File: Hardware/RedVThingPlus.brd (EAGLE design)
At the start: 58.4 x 22.9 mm, 91 parts, among them J1 FEMALE 2x3, J2 USB Female Type C Connector, J5 JTAG, Q1 3.1A/30V/105mΩ, U1 MCP73831, U2 1.8V, U3 AP2112-3.3V, U4 FE310, U5 32MB, Y1 32.768KHZ, Y2 16MHz

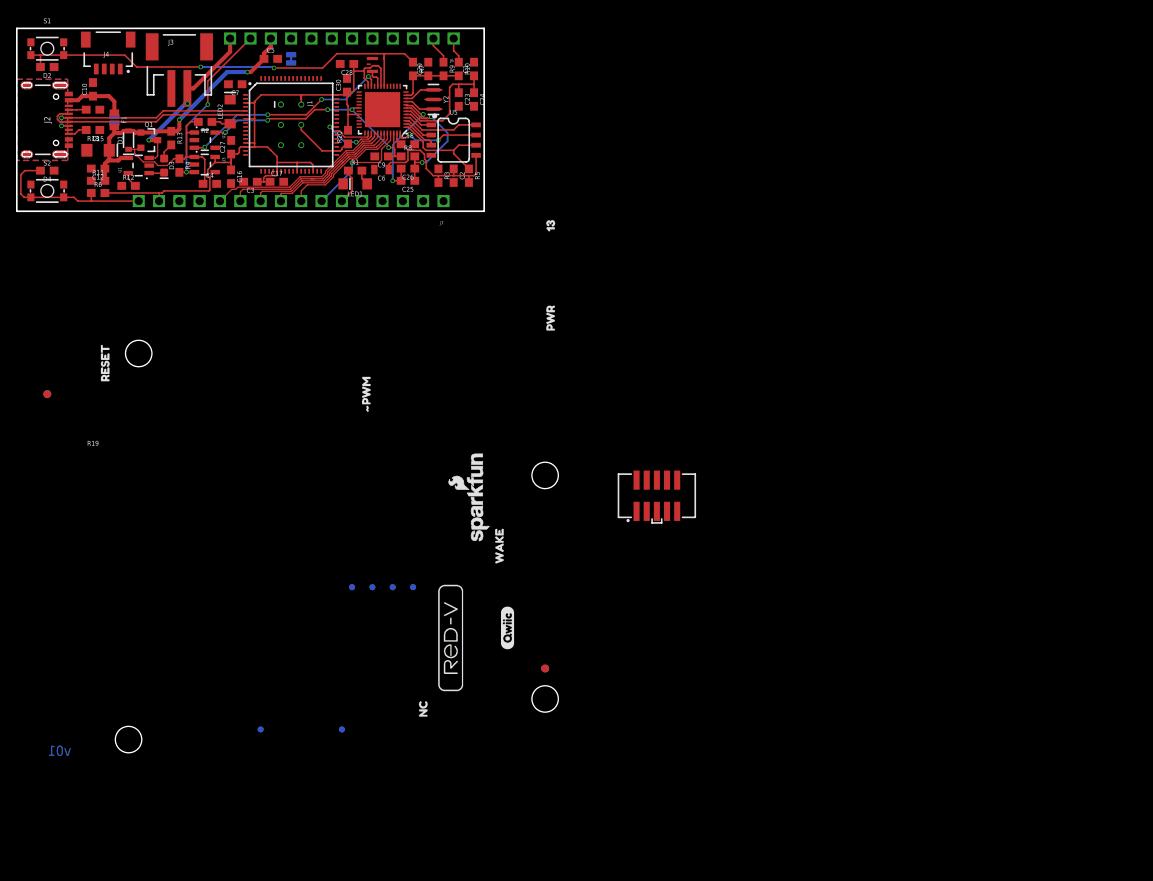
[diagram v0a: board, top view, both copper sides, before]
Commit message: initial layout complete, needs silk
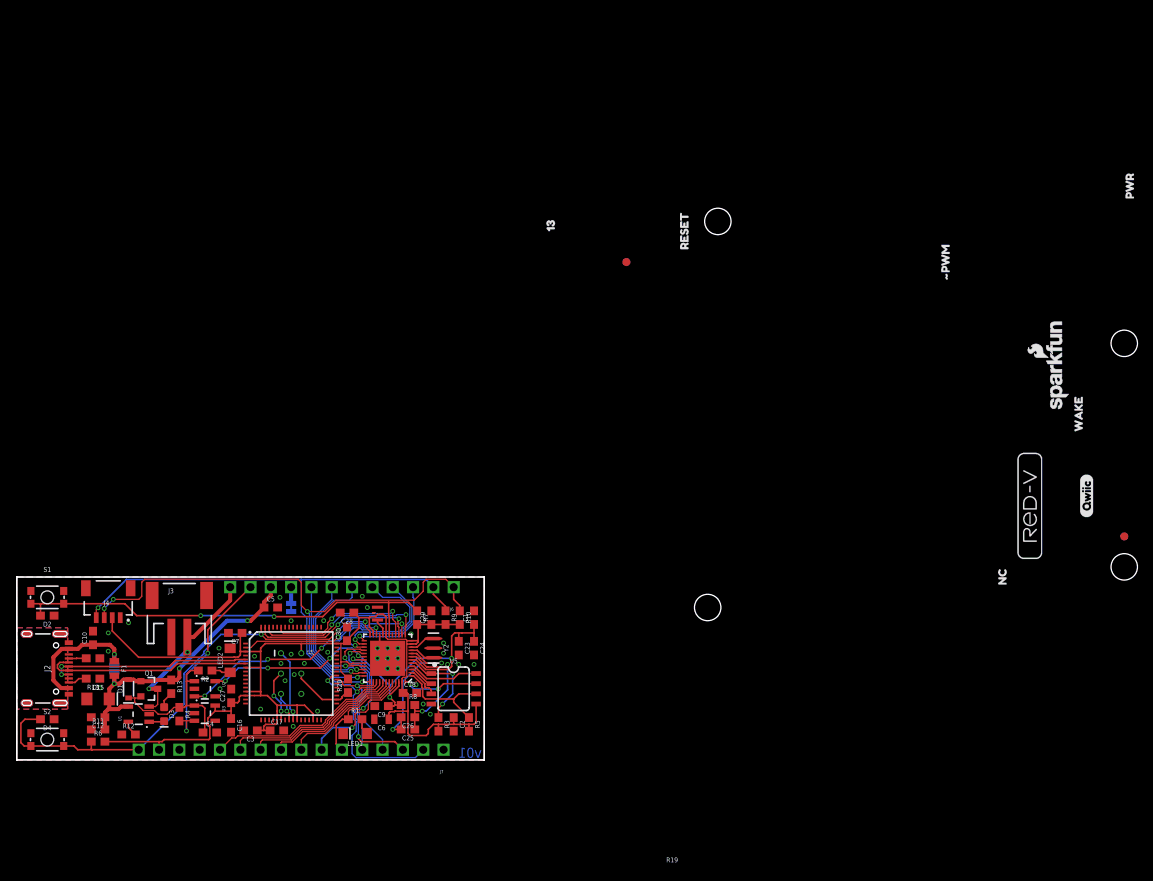
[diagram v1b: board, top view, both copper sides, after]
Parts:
- removed J5: JTAG, SparkFun-Connectors:2X5-SMD-1.27MM
- removed TP1, TP2, TP3, TP4, TP6, TP7: TEST-POINT3, SparkFun-Connectors:PAD.03X.03
- moved JP15 74.2 mm to (76.2, 62.2)
- moved JP16 74.2 mm to (138.4, 27.9)
- moved JP3 74.2 mm to (86.4, 19.1)
- moved JP4 74.2 mm to (138.4, 24.1)
- moved JP5 74.2 mm to (138.4, 52.1)
- moved JP6 74.2 mm to (87.6, 67.3)
- moved JP8 74.2 mm to (138.4, 27.9)
- moved JP9 74.2 mm to (76.2, 62.2)
- moved LOGO1 74.2 mm to (130.0, 49.4)
- moved U$16 74.2 mm to (74.9, 64.8)
- moved U$38 74.2 mm to (123.2, 21.0)
- moved U$42 74.2 mm to (116.1, 58.7)
- moved U$46 74.2 mm to (139.1, 69.2)
- moved U$50 74.2 mm to (132.7, 40.1)
- moved U$52 74.2 mm to (126.6, 31.8)
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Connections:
- net !RESET: no longer J5.10
- net 3.3V: no longer J5.1, TP6.P$1
- net GND: no longer J5.3, J5.5, J5.9, TP7.P$1
- net TCK: no longer J5.4, TP2.P$1
- net TDI: no longer J5.8, TP4.P$1
- net TDO: no longer J5.6, TP3.P$1
- net TMS: no longer J5.2, TP1.P$1
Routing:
- net SDA: track 3.22 -> 70.3 mm, vias 0 -> 4
- net SCL: track 3.49 -> 67.7 mm, vias 0 -> 2
- net !RESET: track 21.2 -> 61.9 mm, vias 0 -> 3
- net 3.3V: track 116.8 -> 154.9 mm
- net TDO: track 0.00 -> 22.4 mm, vias 0 -> 2
- net TCK: track 0.00 -> 21.7 mm, vias 0 -> 2
- net TMS: track 0.00 -> 20.9 mm, vias 0 -> 2
- net IO2: track 0.00 -> 19.4 mm, vias 0 -> 1
- net TDI: track 0.00 -> 19.2 mm, vias 0 -> 2
- net TXO: track 7.55 -> 26.6 mm
- net IO9: track 0.00 -> 17.9 mm, vias 0 -> 1
- net SPI_MISO: track 0.00 -> 17.4 mm, vias 0 -> 1
- net SPI_MOSI: track 0.00 -> 17.3 mm, vias 0 -> 1
- net IO10: track 0.00 -> 16.5 mm, vias 0 -> 1
- net IO11: track 0.00 -> 15.9 mm, vias 0 -> 1
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- added copper zone on layer 1, net GND
- added copper zone on layer 16, net GND

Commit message: v10 changes for Reds design review
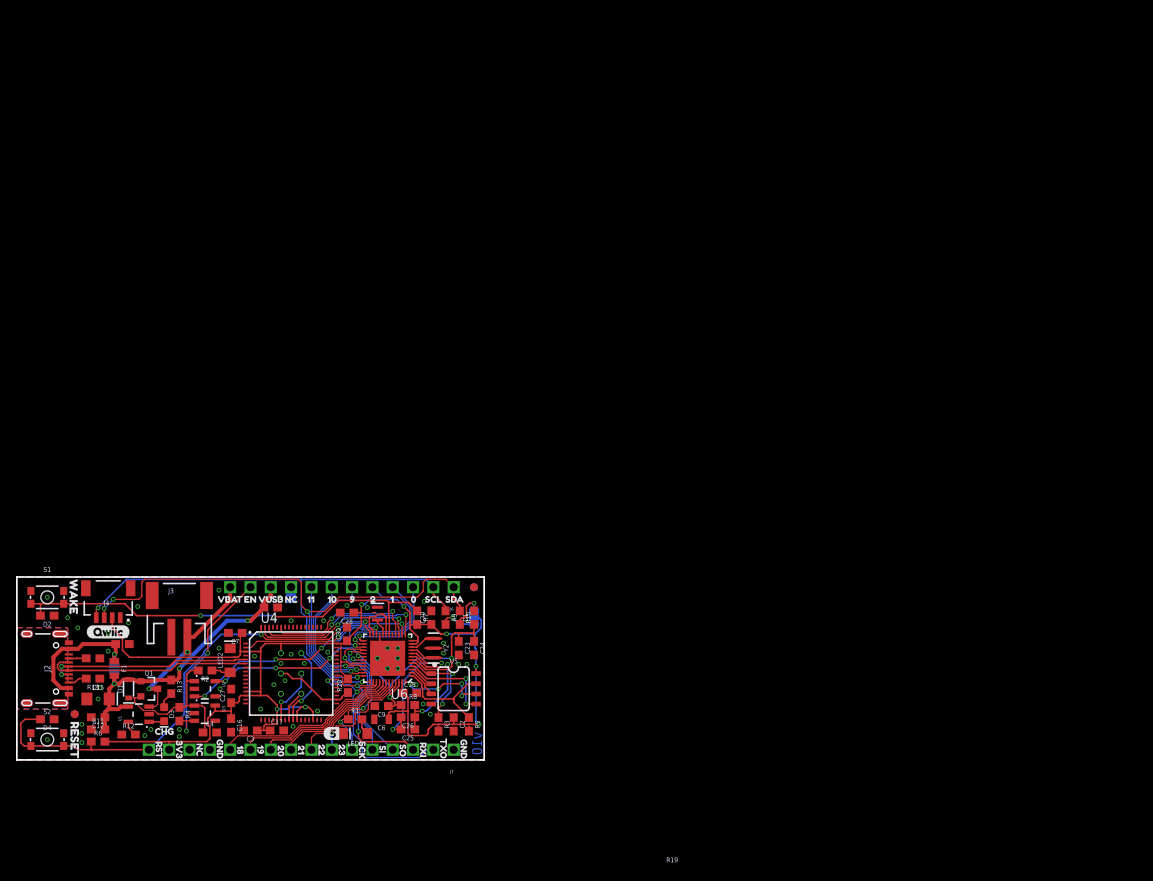
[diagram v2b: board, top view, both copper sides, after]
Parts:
- removed JP1: JUMPER-SMT_2_NC_TRACE_SILK, SparkFun-Jumpers:SMT-JUMPER_2_NC_TRACE_SILK
- removed JP3, JP4, JP5, JP6: STAND-OFF, SparkFun:STAND-OFF
- added I2C: JUMPER-SMT_3_NO_NO-SILK, SparkFun-Jumpers:SMT-JUMPER_3_NO_NO-SILK
- added NC/GND: JUMPER-SMT_2_NO_NO-SILK, SparkFun-Jumpers:SMT-JUMPER_2_NO_NO-SILK
- added U$11: (no value), buzzard_labels (1):118
- added U$12: (no value), buzzard_labels (1):1811
- added U$14: (no value), buzzard_labels (1):1912
- added U$15: (no value), buzzard_labels (1):2013
- added U$17: (no value), buzzard_labels (1):2114
- added U$18: (no value), buzzard_labels (1):2215
- added U$19: (no value), buzzard_labels (1):2316
- added U$2: (no value), buzzard_labels (1):96
- added U$20: (no value), buzzard_labels (1):EN18
- added U$21, U$28: (no value), buzzard_labels (1):GND0
- added U$22, U$27: (no value), buzzard_labels (1):NC17
- added U$23: (no value), buzzard_labels (1):RXI2
- added U$24: (no value), buzzard_labels (1):SCK5
- added U$25: (no value), buzzard_labels (1):SCL10
- added U$26: (no value), buzzard_labels (1):VBAT19
- added U$29: (no value), buzzard_labels (2):#RESET34
- added U$3: (no value), buzzard_labels (2):26
- added U$30: (no value), buzzard_labels (2):3V332
- added U$31: (no value), buzzard_labels (2):3V333
- added U$32: (no value), buzzard_labels (2):015
- added U$33: (no value), buzzard_labels (2):114
- added U$34: (no value), buzzard_labels (2):213
- added U$35: (no value), buzzard_labels (2):912
- added U$36: (no value), buzzard_labels (2):1011
- added U$37: (no value), buzzard_labels (2):1110
- added U$39: (no value), buzzard_labels (2):1828
- added U$4: (no value), buzzard_labels (2):15
- added U$40: (no value), buzzard_labels (2):1927
- added U$41: (no value), buzzard_labels (2):2026
- added U$43: (no value), buzzard_labels (2):2125
- added U$47: (no value), buzzard_labels (2):2323
- added U$48: (no value), buzzard_labels (2):EN8
- added U$5: (no value), buzzard_labels (2):04
- added U$51, U$67: (no value), buzzard_labels (2):GND29
- added U$53: (no value), buzzard_labels (2):MOSI#320
- added U$54: (no value), buzzard_labels (2):NC#GND31
- added U$55: (no value), buzzard_labels (2):NC30
- added U$56: (no value), buzzard_labels (2):RST2
- added U$57: (no value), buzzard_labels (2):RXI#1619
- added U$58: (no value), buzzard_labels (2):SCK#522
- added U$59: (no value), buzzard_labels (2):SCL#1316
- added U$6: (no value), buzzard_labels (1):SDA9
- added U$60: (no value), buzzard_labels (2):SDA#1217
- added U$61: (no value), buzzard_labels (2):SI0
- added U$62: (no value), buzzard_labels (2):SO1
- added U$63: (no value), buzzard_labels (2):TXO#1718
- added U$64: (no value), buzzard_labels (2):VBAT7
- added U$65: (no value), buzzard_labels (2):VUSB3
- added U$66: (no value), buzzard_labels (2):VUSB9
- added U$68: (no value), buzzard_labels (3):RESET1
- added U$69: (no value), buzzard_labels (3):WAKE0
- added U$8: (no value), buzzard_labels (1):TXO1
- added U$9: (no value), buzzard_labels (1):107
- added U6: FE310, SparkFun-IC-Microcontroller:QFN-48-.4MMPITCH
- J4: value (none) -> QWIIC_RIGHT_ANGLE
- U$38: device buzzard_labels (6):NC7 -> buzzard_labels (4):CHG0
- U$42: device buzzard_labels (6):_#PWM30 -> Redfive_logo#04#jpg (3):REDFIVE_LOGO#04#JPG
- U$44: value MK22FN128VLH10 -> (none); device SparkFun-IC-Comms:LQFP-64 -> buzzard_labels (2):2224
- U$45: device buzzard_labels (7):133 -> seggerlogo#png:SEGGERLOGO#PNG
- U$46: device buzzard_labels (7):PWR0 -> buzzard_labels (5):51
- U$49: device buzzard_labels (8):RESET0 -> buzzard_labels (6):THING_PLUS0
- U$50: device buzzard_labels (8):WAKE1 -> buzzard_labels (8):I2C_______0
- U$52: device Redfive_logo#05#png (2):REDFIVE_LOGO#05#PNG -> buzzard_labels (2):MISO#421
- U2: value 1.8V -> AP2127K-1.8V
- U4: value FE310 -> MK22FN128VLH10; device SparkFun-IC-Microcontroller:QFN-48-.4MMPITCH -> SparkFun-IC-Comms:LQFP-64
- U5: value 32MB -> 32MBit
- moved JP16 133.1 mm to (7.24, 5.71)
- moved JP8 133.1 mm to (7.24, 5.71)
- moved U$1 125.9 mm to (8.64, 16.0), turned to 0 degrees
- moved U$46 120.5 mm to (38.2, 3.30), turned to 0 degrees
- moved LOGO1 112.2 mm to (24.5, 11.4), flipped to the bottom
- moved U$38 108.1 mm to (16.5, 3.56), turned to 0 degrees
- moved U$42 105.6 mm to (21.6, 11.6), flipped to the bottom
- moved U$16 90.5 mm to (1.83, 11.4), turned to 90 degrees
- moved U$49 85.3 mm to (19.0, 7.00), flipped to the bottom
- moved U$52 85.2 mm to (47.0, 1.52), flipped to the bottom
- moved U$50 80.3 mm to (57.1, 13.0), flipped to the bottom
- moved U$45 74.5 mm to (10.5, 16.3), flipped to the bottom
- moved JP15 44.9 mm to (57.1, 21.6)
- moved JP9 44.9 mm to (57.1, 21.6)
- moved U4 12.2 mm to (34.3, 10.8), turned to 0 degrees
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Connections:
- new net N$5: I2C.1, R9.2
- new net N$6: I2C.3, R10.2
- net !RESET: now also U4.64, U6.24; no longer U$44.64, U4.24
- net !WAKE: now also U6.18; no longer U4.18
- net 1.8V: now also U6.30, U6.46, U6.6; no longer U4.30, U4.46, U4.6
- net 3.3V: now also I2C.2, U4.13, U4.14, U4.21, U4.26, U4.3, U4.30, U4.48, U4.7, U5.8, U6.11, U6.12, U6.19, U6.23, U6.32, U6.47; no longer R10.2, R9.2, U$44.13, U$44.14, U$44.21, U$44.26, U$44.3, U$44.30, U$44.48, U$44.7, U4.11, U4.12, U4.19, U4.23, U4.32, U4.47, U5.5
- net CORE_ENABLE: now also U6.22; no longer U4.22
- net D+: now also U4.5; no longer U$44.5
- net D-: now also U4.6; no longer U$44.6
- net DBG_RESET: now also U4.34; no longer U$44.34
- net DBG_SWDCLK: now also U4.22; no longer U$44.22
- net DBG_SWDIO: now also U4.25; no longer U$44.25
- net DBG_SWO: now also U4.24; no longer U$44.24
- net GND: now also NC/GND.1, U4.15, U4.16, U4.31, U4.4, U4.47, U6.21, U6.49; no longer J2.SHLD1, J2.SHLD2, J2.SHLD3, J2.SHLD4, J2.SHLD5, J2.SHLD6, J2.SHLD7, J2.SHLD8, JP1.1, U$44.15, U$44.16, U$44.31, U$44.4, U$44.47, U4.21, U4.49
- net IO0: now also U6.25; no longer U4.25
- net IO1: now also U6.26; no longer U4.26
- net IO10: now also U6.34; no longer U4.34
- net IO11: now also U6.35; no longer U4.35
- net IO18: now also U6.40; no longer U4.40
- net IO19: now also U6.41; no longer U4.41
- net IO2: now also U6.27; no longer U4.27
- net IO20: now also U6.42; no longer U4.42
- net IO21: now also U6.43; no longer U4.43
- net IO22: now also U6.44; no longer U4.44
- net IO23: now also U6.45; no longer U4.45
- net IO9: now also U6.33; no longer U4.33
- net N$10: now also U6.8; no longer U4.8
- net N$3: now also U6.10; no longer U4.10
- net N$4: now also NC/GND.2; no longer JP1.2
- net N$7: now also U6.9; no longer U4.9
- net N$8: now also U6.20; no longer U4.20
- net PLL_AVDD: now also U6.7; no longer U4.7
- net QSPI_0: now also U5.5, U6.4; no longer U4.4, U5.8
- net QSPI_1: now also U6.3; no longer U4.3
- net QSPI_2: now also U6.2; no longer U4.2
- net QSPI_3: now also U5.7, U6.1; no longer U4.1, U5.6
- net QSPI_CS: now also U6.5; no longer U4.5
- net QSPI_SCK: now also U5.6, U6.48; no longer U4.48, U5.7
- net RXI: now also U4.40, U6.38; no longer U$44.39, U4.38
- net SCL: now also U6.37; no longer U4.37
- net SDA: now also U6.36; no longer U4.36
- net SPI_MISO: now also U6.29; no longer U4.29
- net SPI_MOSI: now also U6.28; no longer U4.28
- net SPI_SCK: now also U6.31; no longer U4.31
- net TCK: now also U4.62, U6.13; no longer U$44.62, U4.13
- net TDI: now also U4.59, U6.16; no longer U$44.59, U4.16
- net TDO: now also U4.2, U6.14; no longer U$44.2, U4.14
- net TMS: now also U4.63, U6.15; no longer U$44.63, U4.15
- net TXO: now also U6.39; no longer U$44.40
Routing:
- net 3.3V: track 154.9 -> 174.4 mm, vias 0 -> 7
- net N$6: track 0.00 -> 4.91 mm, vias 0 -> 1
- net N$5: track 0.00 -> 4.59 mm, vias 0 -> 1
- net QSPI_0: track 9.03 -> 12.0 mm, vias 0 -> 2
- net RXI: track 19.2 -> 21.4 mm
- net GND: track 2.38 -> 4.61 mm, vias 37 -> 50
- net DBG_RESET: track 8.00 -> 10.2 mm
- net QSPI_SCK: track 9.65 -> 11.3 mm, vias 2 -> 4
- net IO21: track 18.0 -> 16.7 mm
- net N$4: track 2.03 -> 0.86 mm
- net IO19: track 22.5 -> 21.4 mm
- net DBG_SWDIO: track 8.97 -> 10.0 mm
- net IO22: track 16.1 -> 15.2 mm
- net !RESET: track 61.9 -> 62.8 mm
- net IO20: track 20.3 -> 19.5 mm
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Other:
- board text added: "v10"
- board text removed: "Based on Arduino by: M. Banzi, D. Cuartielles, T. Igoe, G. Martino, D. Mellis"
- board text removed: "v01"
